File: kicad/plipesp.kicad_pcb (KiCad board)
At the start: 2 copper layers, 38 x 35.5 mm, 37 parts, among them CON1 IEEEE-1284A, J1 USB_B_Micro, J2 Conn_01x04_Male, J3 Conn_01x06_Male, J4 Micro_SD_Card_Det, U1 AMS1117-3.3, U2 CBTD3384, U3 CBTD3384, U4 ESP32-WROOM-32D

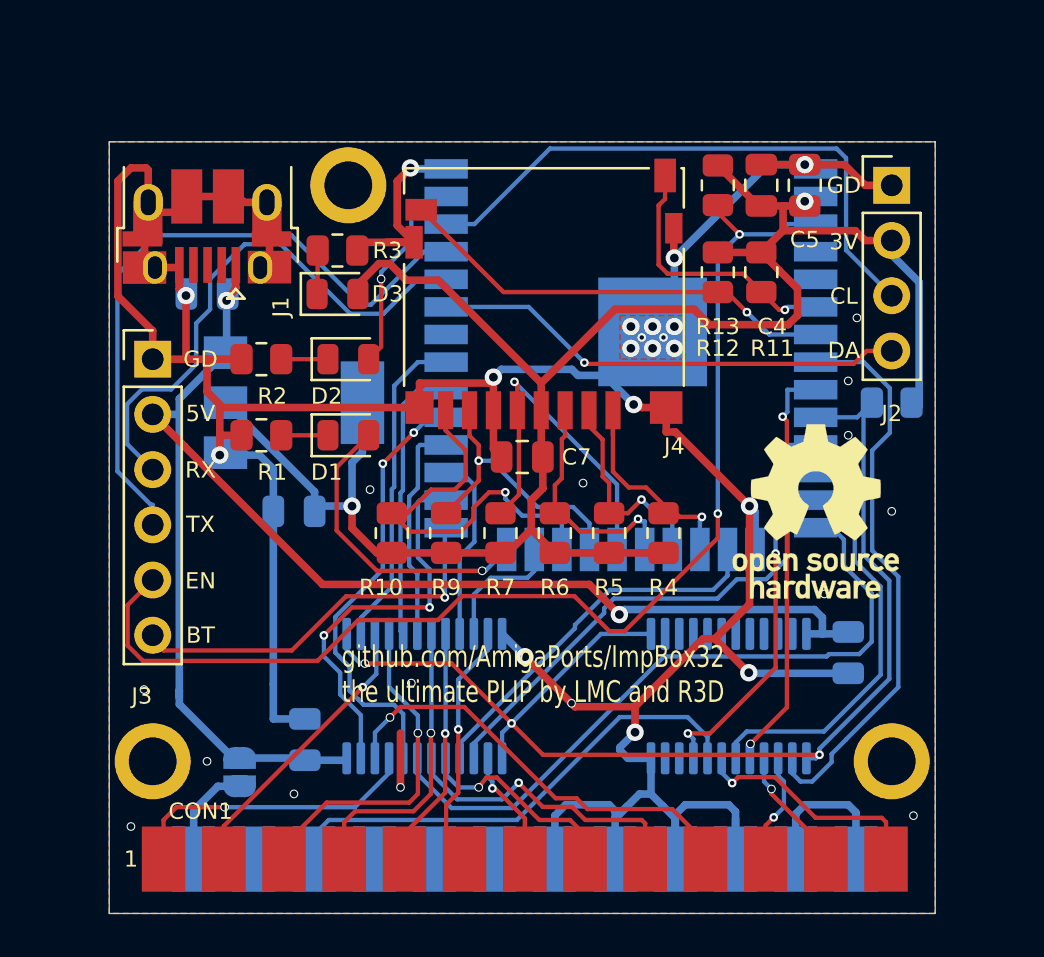
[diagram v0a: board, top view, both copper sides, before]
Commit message: board rev2
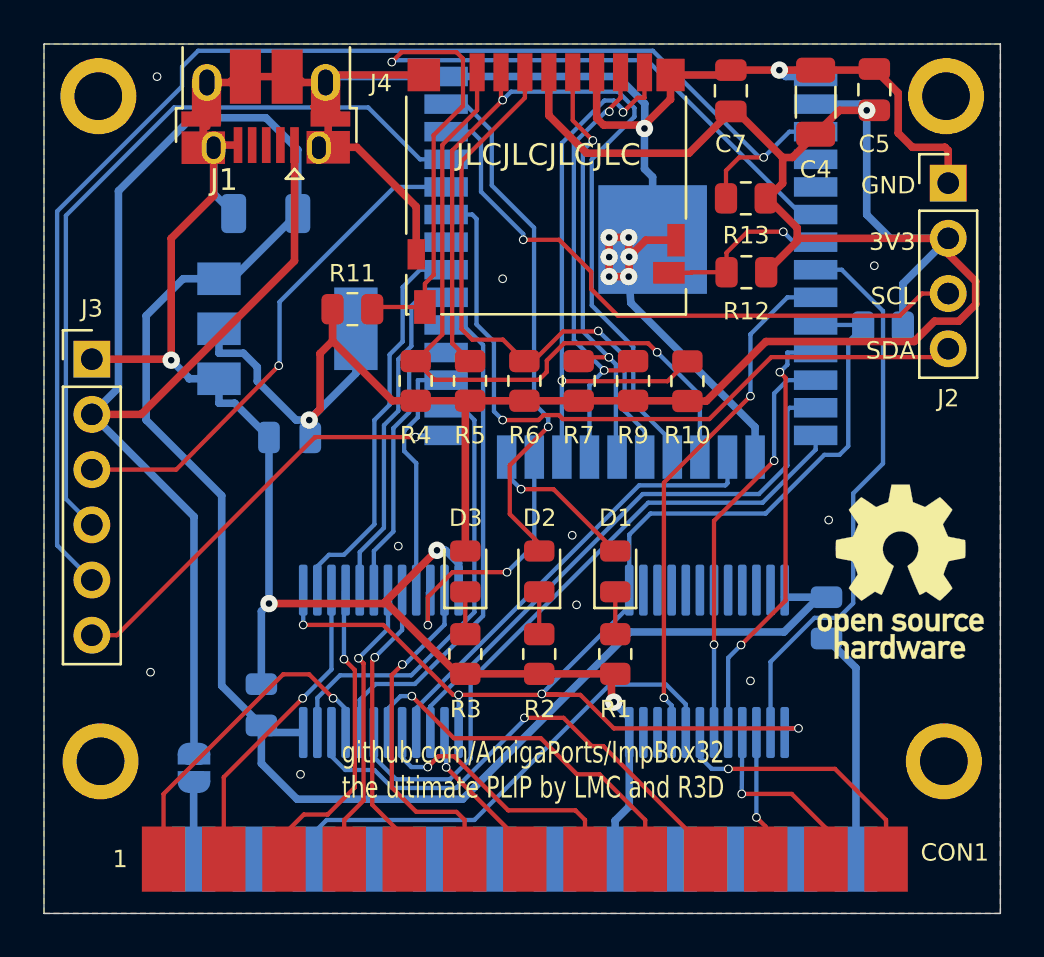
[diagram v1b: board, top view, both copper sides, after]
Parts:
- added REF4: mounting_hole, plipesp:mounting_hole, F.Cu at (123.0, 127.3)
- C3, C4: footprint Capacitor_SMD:C_0805_2012Metric -> Capacitor_SMD:C_1206_3216Metric
- J1: footprint Connector_USB:USB_Micro-B_Amphenol_10103594-0001LF_Horizontal -> plipesp:USB_Micro-B_Amphenol_10103594-0001LF_Horizontal
- U2, U3: footprint Package_SO:TSSOP-24_4.4x7.8mm_P0.65mm -> plipesp:SO-universal-24_P0.65mm
- U4: footprint RF_Module:ESP32-WROOM-32 -> plipesp:ESP32-WROOM-32
- moved R3 19.5 mm to (100.9, 153.0), turned to -90 degrees
- moved C7 19.4 mm to (113.1, 127.0), turned to 90 degrees
- moved R1 19.1 mm to (107.8, 153.0), turned to -90 degrees
- moved R11 18.9 mm to (95.7, 137.1), turned to 0 degrees
- moved R2 18.6 mm to (104.3, 153.0), turned to -90 degrees
- moved R10 15.3 mm to (111.1, 140.4)
- moved D3 14.1 mm to (100.9, 149.2), turned to 90 degrees
- moved D1 13.8 mm to (107.8, 149.2), turned to 90 degrees
- moved R4 13.4 mm to (98.6, 140.4)
- moved D2 13.1 mm to (104.3, 149.2), turned to 90 degrees
- moved REF1 12.2 mm to (84.0, 127.3)
- moved R9 11.1 mm to (108.6, 140.4)
- moved R5 9.48 mm to (101.1, 140.4)
- moved R7 7.87 mm to (106.1, 140.4)
- moved R6 7.14 mm to (103.6, 140.4)
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- renumbered REF** to REF1, REF** to REF2, REF** to REF3
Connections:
- net ~ACK renamed ~{ACK}
- net ~IO_EN renamed ~{IO_EN}
- net ~SD_DETECT1 renamed ~{SD_DETECT1}
- net ~SD_DETECT2 renamed ~{SD_DETECT2}
- net ~STROBE renamed ~{STROBE}
- CON1 pad 15: Net-(CON1-Pad15) -> unconnected-(CON1-Pad15)
- J1 pad 2: Net-(J1-Pad2) -> unconnected-(J1-Pad2)
- J1 pad 3: Net-(J1-Pad3) -> unconnected-(J1-Pad3)
- J1 pad 4: Net-(J1-Pad4) -> unconnected-(J1-Pad4)
- U3 pad 10: Net-(U3-Pad10) -> unconnected-(U3-Pad10)
- U3 pad 11: Net-(U3-Pad11) -> unconnected-(U3-Pad11)
- U3 pad 14: Net-(U3-Pad14) -> unconnected-(U3-Pad14)
- U3 pad 15: Net-(U3-Pad15) -> unconnected-(U3-Pad15)
- U3 pad 16: Net-(U3-Pad16) -> unconnected-(U3-Pad16)
- U3 pad 17: Net-(U3-Pad17) -> unconnected-(U3-Pad17)
- U3 pad 18: Net-(U3-Pad18) -> unconnected-(U3-Pad18)
- U3 pad 19: Net-(U3-Pad19) -> unconnected-(U3-Pad19)
- U3 pad 20: Net-(U3-Pad20) -> unconnected-(U3-Pad20)
- U3 pad 21: Net-(U3-Pad21) -> unconnected-(U3-Pad21)
- U3 pad 22: Net-(U3-Pad22) -> unconnected-(U3-Pad22)
- U3 pad 23: Net-(U3-Pad23) -> unconnected-(U3-Pad23)
- U3 pad 9: ~AMI_RESET -> ~{AMI_RESET}
- U4 pad 11: ~AMI_RESET -> POUT
- U4 pad 32: Net-(U4-Pad32) -> unconnected-(U4-Pad32)
- U4 pad 4: Net-(U4-Pad4) -> unconnected-(U4-Pad4)
- U4 pad 5: Net-(U4-Pad5) -> unconnected-(U4-Pad5)
- U4 pad 9: POUT -> ~{AMI_RESET}
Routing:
- net +5V: track 69.5 -> 123.9 mm, vias 2 -> 0
- net SD_D3: track 10.00 -> 38.9 mm
- net ~{SD_DETECT1}: track 12.4 -> 39.5 mm
- net ~{AMI_RESET}: track 0.00 -> 23.8 mm, vias 0 -> 2
- net SD_D2: track 11.0 -> 32.7 mm
- net +3V3: track 89.9 -> 110.8 mm
- net ~AMI_RESET: track 18.3 -> 0.00 mm, vias 2 -> 0
- net SD_CMD: track 11.0 -> 26.8 mm
- net LED_STATUS2: track 9.38 -> 23.1 mm
- net ~{SD_DETECT2}: track 20.5 -> 8.26 mm
- net GND: track 198.3 -> 186.6 mm, vias 34 -> 22
- net I2C_SDA: track 21.8 -> 33.2 mm
- net SD_D1: track 18.8 -> 27.0 mm, vias 1 -> 2
- net SD_D0: track 13.0 -> 21.1 mm, vias 1 -> 2
- net LED_STATUS: track 14.0 -> 6.45 mm
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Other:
- board size 38 x 35.5 mm -> 44 x 40 mm
- net class Default removed
- net class power removed
- board text added: "3V3"
- board text added: "GND"
- board text added: "JLCJLCJLCJLC"
- board text added: "Rock n Roll doctor Rev. 2"
- board text added: "SCL"
- board text added: "SDA"
- board text removed: "3V"
- board text removed: "CL"
- board text removed: "DA"
- board text removed: "GD"
- board text removed: "Rock n Roll doctor Rev. 1"
